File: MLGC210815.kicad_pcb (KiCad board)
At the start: 2 copper layers, 8 parts, among them J1 PinStrip_01x06_Male, U1 PIC32MM0064GPL028-I_SO

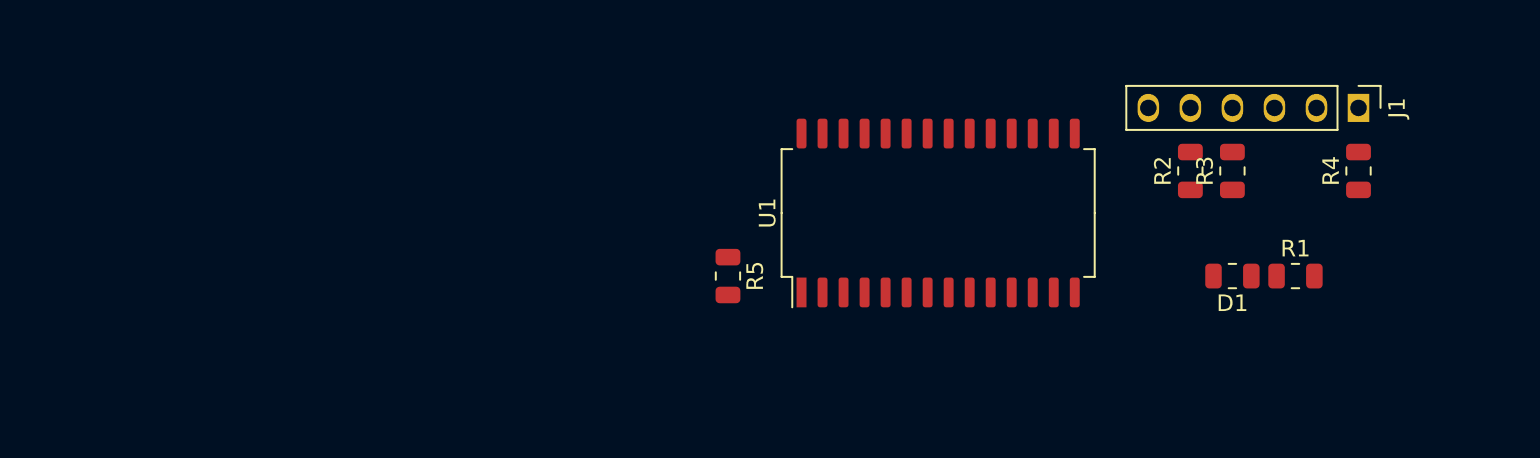
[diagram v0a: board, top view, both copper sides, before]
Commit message: update
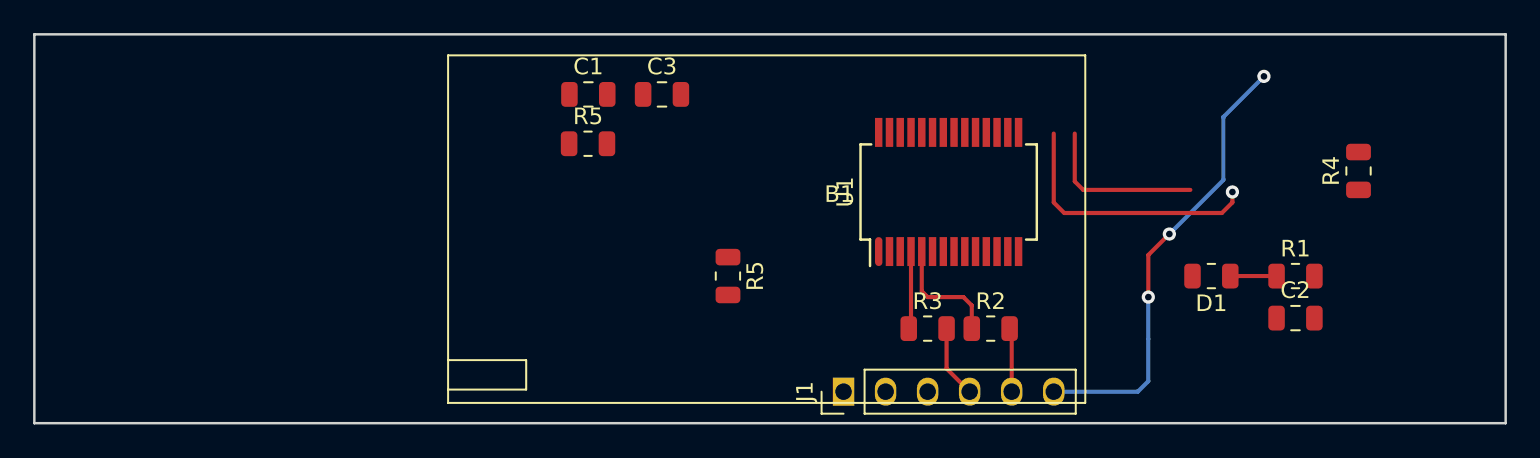
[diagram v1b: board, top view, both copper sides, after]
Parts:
- added B1: L402036, Others:Battery_L402036, F.Cu at (143.5, 70.5)
- added C1: C0805_100nF, Passive:C0805, F.Cu at (113.5, 72.8)
- added C2: C0805_100nF, Passive:C0805, F.Cu at (156.2, 86.4)
- added C3: C0805_10uF, Passive:C0805, F.Cu at (117.9, 72.8)
- added R5: R0805_4K70, Passive:R0805, F.Cu at (113.5, 75.8)
- U1: value PIC32MM0064GPL028-I_SO -> PIC32MX170F256B-ISS; footprint Integrated Circuits:SOIC-28W -> Integrated Circuits:SSOP-28
- moved J1 35.5 mm to (128.9, 90.8), turned to 90 degrees
- moved R3 20.7 mm to (134.0, 87.0), turned to 0 degrees
- moved R2 15.4 mm to (137.8, 87.0), turned to 0 degrees
- moved U1 1.42 mm to (135.3, 78.7)
- moved D1 1.27 mm to (151.1, 83.8)
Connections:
- net Net-(U1-Pad17) renamed /SCL
- net Net-(U1-Pad6) renamed /IC1
- J1 pad 2: GND -> +3V3
- J1 pad 3: +3V3 -> GND
- R2 pad 1: /PGC-RB6 -> /PGC
- R3 pad 1: /PGD-RB7 -> /PGD
- U1 pad 13: Net-(U1-Pad13) -> +3V3
- U1 pad 15: /PGC-RB6 -> Net-(U1-Pad15)
- U1 pad 16: /PGD-RB7 -> /SDA
- U1 pad 27: Net-(U1-Pad27) -> GND
- U1 pad 28: Net-(U1-Pad28) -> +3V3
- U1 pad 4: Net-(U1-Pad4) -> /PGD
- U1 pad 5: Net-(U1-Pad5) -> /PGC
- U1 pad 8: Net-(U1-Pad8) -> GND
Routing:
- net Net-(J1-Pad6): track 0.00 -> 27.3 mm, vias 0 -> 3
- net /PGD: track 0.00 -> 21.0 mm, vias 0 -> 1
- net /PGC: track 0.00 -> 17.3 mm
- net Net-(J1-Pad4): track 0.00 -> 5.02 mm
- net Net-(J1-Pad5): track 0.00 -> 3.86 mm
- net Net-(D1-Pad1): track 0.00 -> 2.79 mm
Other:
- board outline added: 88.9 x 23.5 mm
